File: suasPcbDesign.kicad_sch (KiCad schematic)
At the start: 95 parts, among them J1 SENSE_IB, J2 SPI CS, J4 SPI CTRL, J5 PWM CTRL, J6 JTAG Pinout, J7 USB_C_Receptacle_USB2.0_16P, SW1 SW_SPST, SW2 SW_SPST, SW3 SW_SPST, SW4 SW_SPST, SW5 SW_SPST, SW6 SW_SPST, SW7 SW_SPST, U1 74HC138, U2 LMR51625DDC, U3 MCP3562RT-E/ST, U4 MCP6486R, U5 TLV77733PDBVR, U6 MCP6541UT-E/OT, U7 ESP32-S3-WROOM-1, U8 LM66100DCK, U9 USBLC6-2SC6

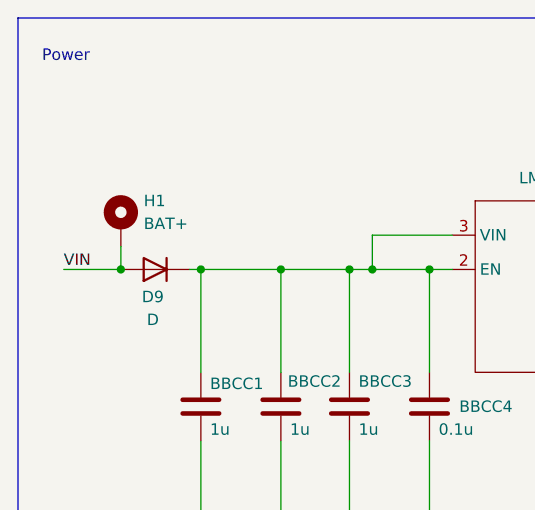
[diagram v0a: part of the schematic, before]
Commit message: Fix diode position
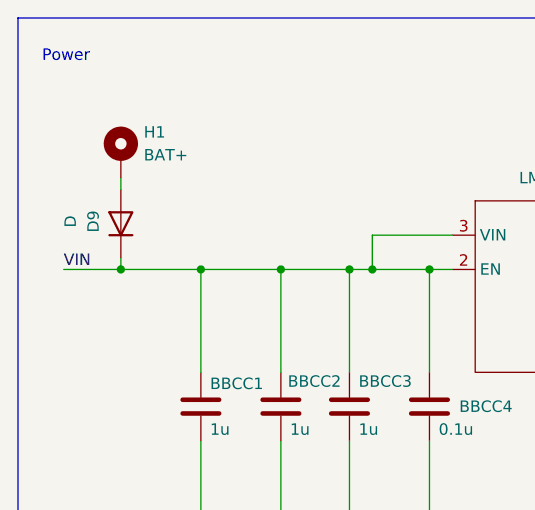
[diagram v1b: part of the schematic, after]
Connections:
- net VIN: now also BBCC1.1, BBCC2.1, BBCC3.1, BBCC4.1, D9.1 (K), U2.2 (EN), U2.3 (VIN); no longer D9.2 (A), H1.1
- new net: D9.2 (A), H1.1
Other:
- moved on the sheet: D9, H1
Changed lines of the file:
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@@
 	)
 	(junction
+		(at 27.94 44.45)
+		(diameter 0)
+		(color 0 0 0 0)
+	)
+	(junction
 		(at 52.07 196.85)
 		(diameter 0)
@@
 	)
 	(junction
-		(at 27.94 44.45)
-		(diameter 0)
-		(color 0 0 0 0)
-	)
-	(junction
 		(at 153.67 102.87)
 		(diameter 0)
@@
 	(wire
 		(pts
-			(xy 35.56 44.45) (xy 36.83 44.45)
-		)
-		(stroke
-			(width 0)
-			(type default)
-		)
-	)
-	(wire
-		(pts
 			(xy 190.5 63.5) (xy 190.5 66.04)
 		)
@@
 	(wire
 		(pts
-			(xy 27.94 41.91) (xy 27.94 44.45)
-		)
-		(stroke
-			(width 0)
-			(type default)
-		)
-	)
-	(wire
-		(pts
 			(xy 87.63 200.66) (xy 87.63 209.55)
 		)
@@
 	(wire
 		(pts
+			(xy 27.94 44.45) (xy 36.83 44.45)
+		)
+		(stroke
+			(width 0)
+			(type default)
+		)
+	)
+	(wire
+		(pts
 			(xy 276.86 186.69) (xy 276.86 187.96)
 		)
@@
 	(wire
 		(pts
+			(xy 27.94 43.18) (xy 27.94 44.45)
+		)
+		(stroke
+			(width 0)
+			(type default)
+		)
+	)
+	(wire
+		(pts
+			(xy 27.94 34.29) (xy 27.94 35.56)
+		)
+		(stroke
+			(width 0)
+			(type default)
+		)
+	)
+	(wire
+		(pts
 			(xy 245.11 71.12) (xy 245.11 73.66)
 		)
@@
 	(symbol
 		(lib_id "Device:D")
-		(at 31.75 44.45 180)
+		(at 27.94 39.37 90)
 		(unit 1)
 		(body_style 1)
@@
 		(dnp no)
 		(property "Reference" "D9"
-			(at 31.496 47.498 0)
+			(at 24.892 39.116 0)
 			(show_name no)
 			(do_not_autoplace no)
@@
 		)
 		(property "Value" "D"
-			(at 31.496 50.038 0)
+			(at 22.352 39.116 0)
 			(show_name no)
 			(do_not_autoplace no)
@@
 		)
 		(property "Footprint" "Diode_SMD:D_SMA-SMB_Universal_Handsoldering"
-			(at 31.75 44.45 0)
+			(at 27.94 39.37 0)
 			(hide yes)
 			(show_name no)
@@
 		)
 		(property "Datasheet" "https://mm.digikey.com/Volume0/opasdata/d220001/medias/docus/6956/5399_S3M%20SMB.pdf"
-			(at 31.75 44.45 0)
+			(at 27.94 39.37 0)
 			(hide yes)
 			(show_name no)
@@
 		)
 		(property "Description" "Diode 5399-S3MCT-ND"
-			(at 31.75 44.45 0)
+			(at 27.94 39.37 0)
 			(hide yes)
 			(show_name no)
@@
 		)
 		(property "Sim.Device" "D"
-			(at 31.75 44.45 0)
+			(at 27.94 39.37 0)
 			(hide yes)
 			(show_name no)
@@
 		)
 		(property "Sim.Pins" "1=K 2=A"
-			(at 31.75 44.45 0)
+			(at 27.94 39.37 0)
 			(hide yes)
 			(show_name no)
@@
 	(symbol
 		(lib_id "Mechanical:MountingHole_Pad")
-		(at 27.94 39.37 0)
+		(at 27.94 31.75 0)
 		(unit 1)
 		(body_style 1)
@@
 		(fields_autoplaced yes)
 		(property "Reference" "H1"
-			(at 30.48 36.8299 0)
+			(at 30.48 29.2099 0)
 			(show_name no)
 			(do_not_autoplace no)
@@
 		)
 		(property "Value" "BAT+"
-			(at 30.48 39.3699 0)
+			(at 30.48 31.7499 0)
 			(show_name no)
 			(do_not_autoplace no)
@@
 		)
 		(property "Footprint" "Custom:7770 Keystone Electronics PC SCREW TERMINALS"
-			(at 27.94 39.37 0)
+			(at 27.94 31.75 0)
 			(hide yes)
 			(show_name no)
@@
 		)
 		(property "Datasheet" ""
-			(at 27.94 39.37 0)
+			(at 27.94 31.75 0)
 			(hide yes)
 			(show_name no)
@@
 		)
 		(property "Description" "Mounting Hole with connection"
-			(at 27.94 39.37 0)
+			(at 27.94 31.75 0)
 			(hide yes)
 			(show_name no)
